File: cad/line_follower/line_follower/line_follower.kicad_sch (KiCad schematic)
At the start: 15 parts

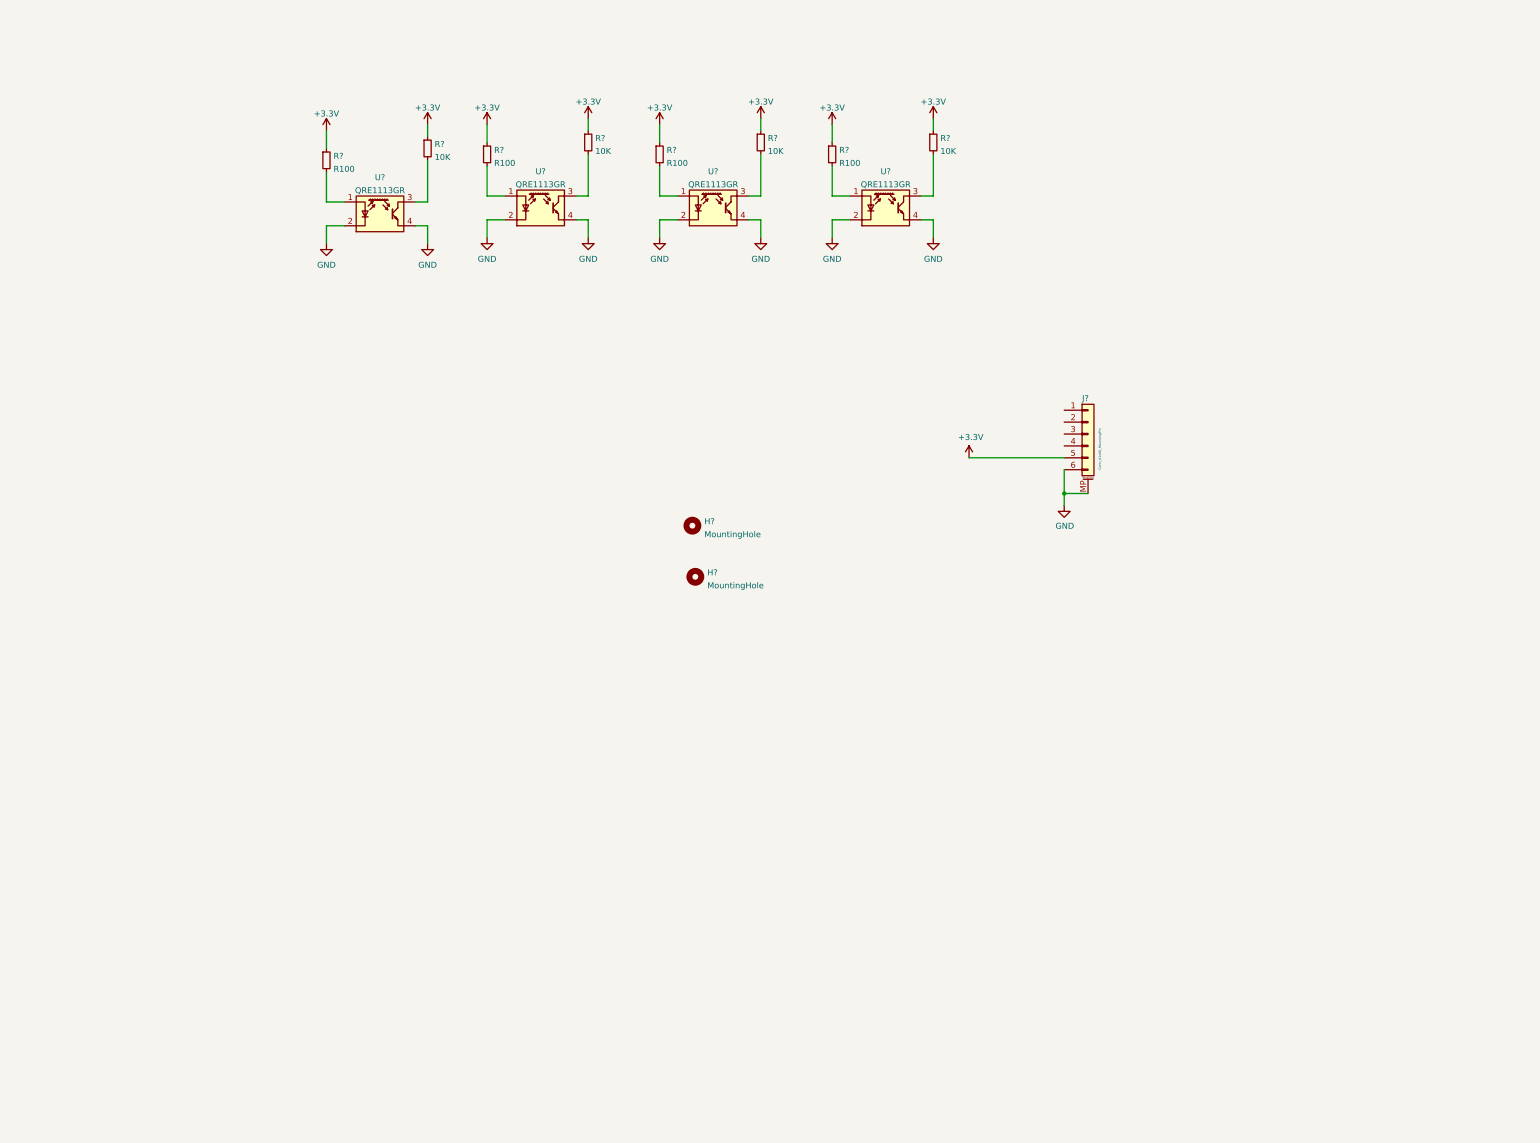
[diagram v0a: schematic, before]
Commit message: Andrew wants what!?!?! 5 more boards???
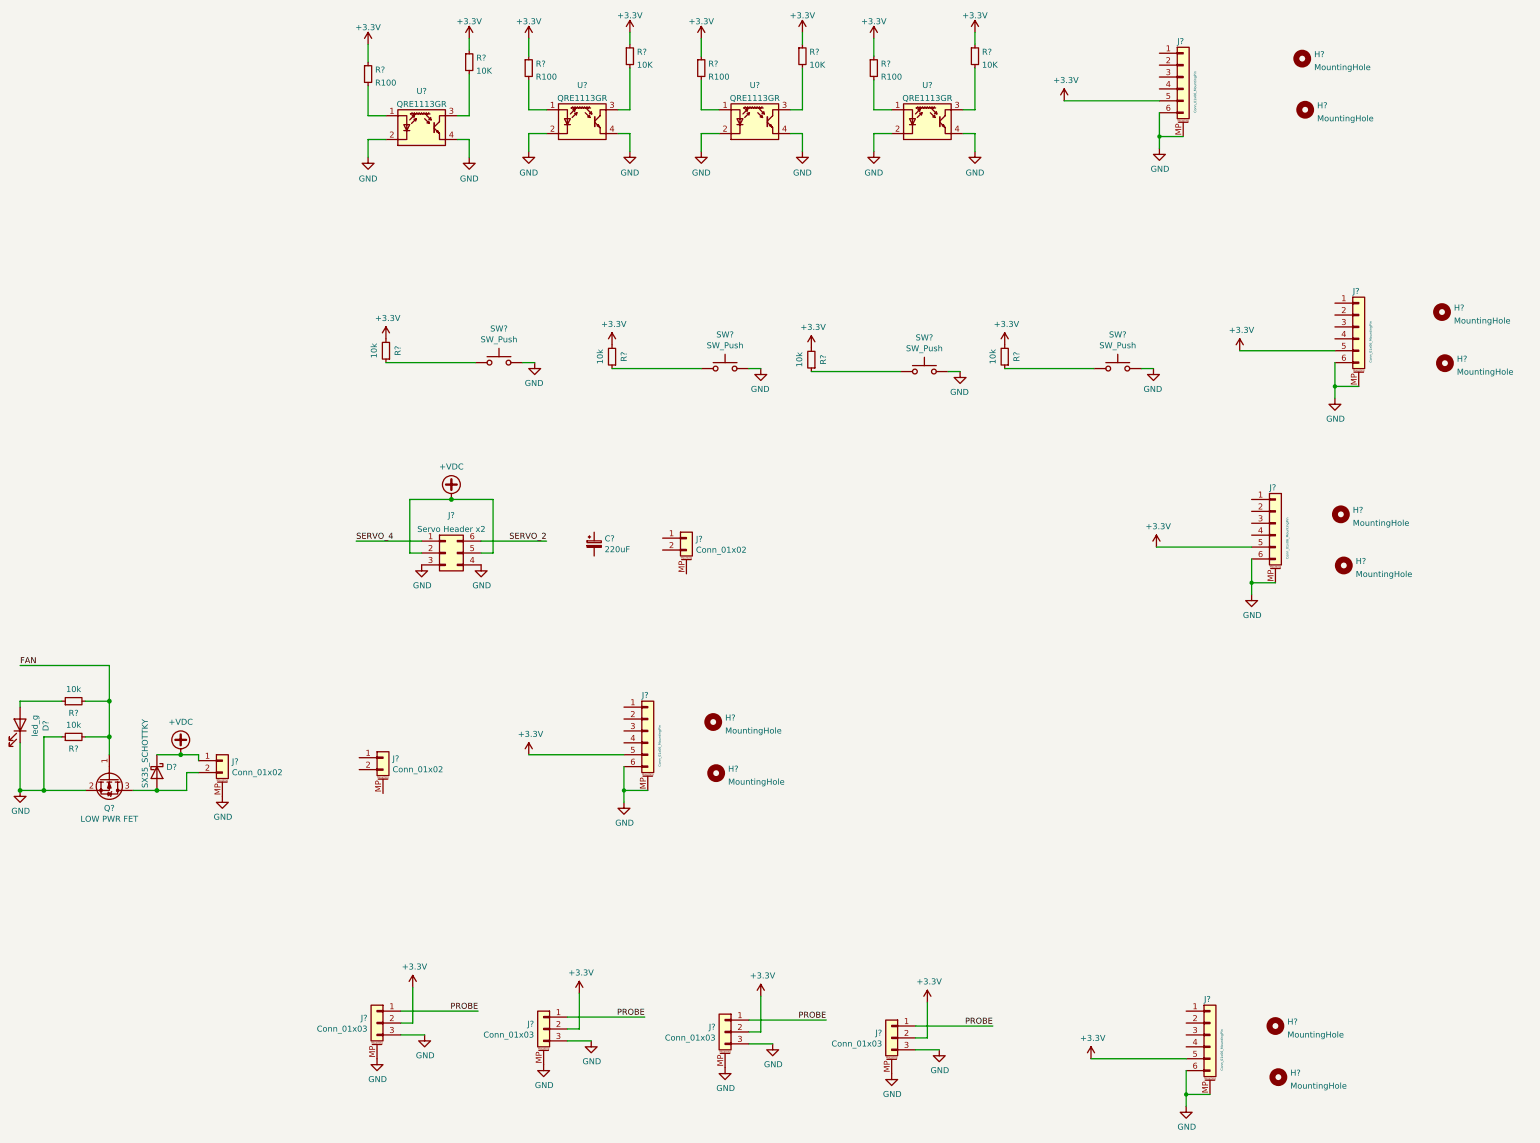
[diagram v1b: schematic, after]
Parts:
- added C?: 220uF, Capacitor_SMD:CP_Elec_10x12.5, symbol Device:CP_Small
- added D?: led_g, LED_SMD:LED_0603_1608Metric, symbol Device:LED
- added D?: SX35_SCHOTTKY, Diode_SMD:D_SMA, symbol Device:D_Schottky
- added H? (x8): MountingHole, MountingHole:MountingHole_3.2mm_M3_ISO14580, symbol Mechanical:MountingHole
- added J? (x4): Conn_01x03, Connector_JST:JST_PH_B3B-PH-SM4-TB_1x03-1MP_P2.00mm_Vertical, symbol Connector_Generic_MountingPin:Conn_01x03_MountingPin
- added J?: Servo Header x2, Evezor_extras:PinHeader_2x03_P2.54mm_Vertical_SMD, symbol Connector_Generic:Conn_02x03_Counter_Clockwise
- added J? (x4): Conn_01x06_MountingPin, Connector_FFC-FPC:TE_84952-6_1x06-1MP_P1.0mm_Horizontal, symbol Connector_Generic_MountingPin:Conn_01x06_MountingPin
- added J? (x3): Conn_01x02, Evezor_extras:CONN_JST_XH_2_VERTICAL, symbol Connector_Generic_MountingPin:Conn_01x02_MountingPin
- added Q?: LOW PWR FET, Package_TO_SOT_SMD:SOT-23, symbol Device:Q_NMOS_GSD
- added R? (x6): 10k, Resistor_SMD:R_0603_1608Metric, symbol Device:R_Small
- added SW? (x4): SW_Push, EvezorLIB:SWITCH_2x3_SMD_TACTILE_GREEN, symbol Switch:SW_Push
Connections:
- net +3V3: now also J?.2 (Pin_2), J?.2 (Pin_2), J?.2 (Pin_2), J?.2 (Pin_2), J?.5 (Pin_5), J?.5 (Pin_5), J?.5 (Pin_5), J?.5 (Pin_5), R?.2, R?.2, R?.2, R?.2
- net GND: now also D?.1 (K), J?.3 (Pin_3), J?.3 (Pin_3), J?.3 (Pin_3), J?.3 (Pin_3), J?.3 (Pin_3), J?.4 (Pin_4), J?.6 (Pin_6), J?.6 (Pin_6), J?.6 (Pin_6), J?.6 (Pin_6), J?.MP (MountPin), J?.MP (MountPin), J?.MP (MountPin), J?.MP (MountPin), J?.MP (MountPin), J?.MP (MountPin), J?.MP (MountPin), J?.MP (MountPin), J?.MP (MountPin), Q?.2 (S), R?.1, SW?.2, SW?.2, SW?.2, SW?.2
- new net: R?.1, SW?.1 (x4)
- new net: D?.2 (A), R?.1
- new net: D?.2 (A), J?.2 (Pin_2), Q?.3 (D)
- new net +VDC: D?.1 (K), J?.1 (Pin_1), J?.2 (Pin_2), J?.5 (Pin_5)
- new net FAN: Q?.1 (G), R?.2, R?.2
- new net PROBE: J?.1 (Pin_1), J?.1 (Pin_1), J?.1 (Pin_1), J?.1 (Pin_1)
- new net SERVO_2: J?.6 (Pin_6)
- new net SERVO_4: J?.1 (Pin_1)
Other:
- moved on the sheet: H?, J?, R?, U?

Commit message: Half of the 2nd floor built, remodeling in progress
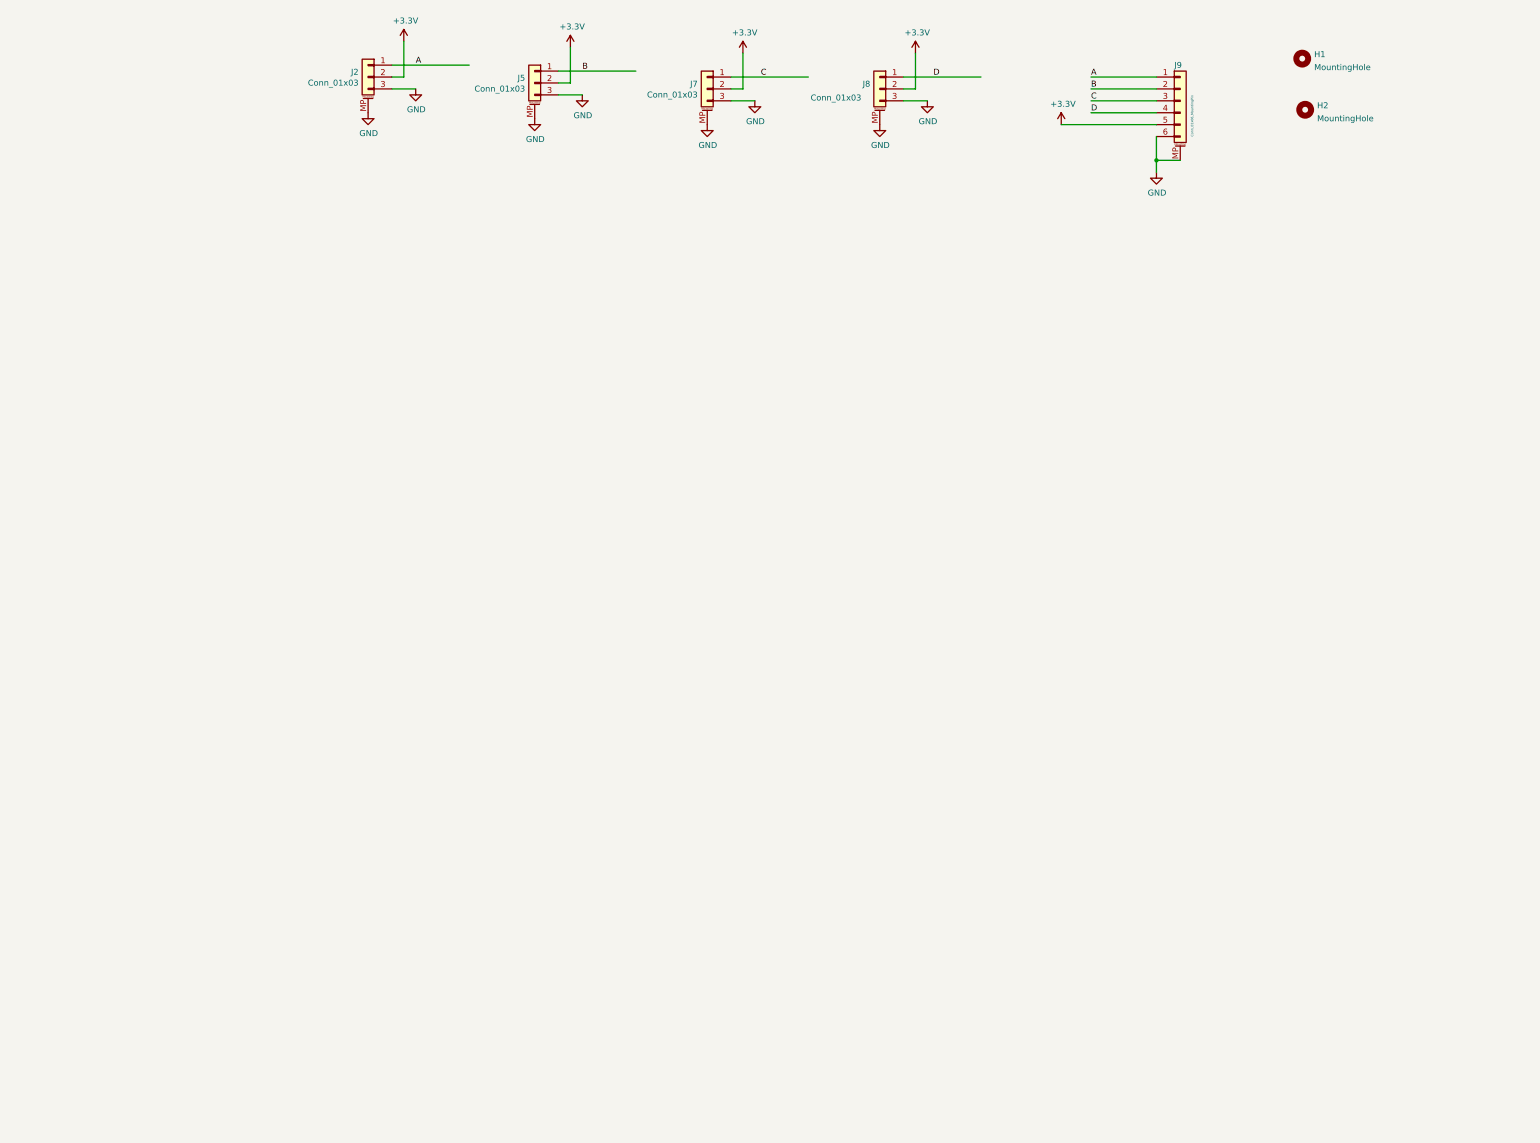
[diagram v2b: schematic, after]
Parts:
- removed C?: 220uF, Capacitor_SMD:CP_Elec_10x12.5, symbol Device:CP_Small
- removed D?: led_g, LED_SMD:LED_0603_1608Metric, symbol Device:LED
- removed D?: SX35_SCHOTTKY, Diode_SMD:D_SMA, symbol Device:D_Schottky
- removed H? (x8): MountingHole, MountingHole:MountingHole_3.2mm_M3_ISO14580, symbol Mechanical:MountingHole
- removed J?: Servo Header x2, Evezor_extras:PinHeader_2x03_P2.54mm_Vertical_SMD, symbol Connector_Generic:Conn_02x03_Counter_Clockwise
- removed J? (x4): Conn_01x06_MountingPin, Connector_FFC-FPC:TE_84952-6_1x06-1MP_P1.0mm_Horizontal, symbol Connector_Generic_MountingPin:Conn_01x06_MountingPin
- removed J? (x3): Conn_01x02, Evezor_extras:CONN_JST_XH_2_VERTICAL, symbol Connector_Generic_MountingPin:Conn_01x02_MountingPin
- removed Q?: LOW PWR FET, Package_TO_SOT_SMD:SOT-23, symbol Device:Q_NMOS_GSD
- removed R? (x6): 10k, Resistor_SMD:R_0603_1608Metric, symbol Device:R_Small
- removed R? (x4): 10K, Resistor_SMD:R_0603_1608Metric, symbol Device:R_Small
- removed R? (x4): R100, Resistor_SMD:R_0603_1608Metric, symbol Device:R_Small
- removed SW? (x4): SW_Push, EvezorLIB:SWITCH_2x3_SMD_TACTILE_GREEN, symbol Switch:SW_Push
- removed U? (x4): QRE1113GR, OptoDevice:OnSemi_CASE100CY, symbol Sensor_Proximity:QRE1113
- gave numbers to parts that had none: 7
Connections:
- net A: now reaches J9.1 (Pin_1)
- net A: now also J2.1 (Pin_1)
- net B: now reaches J9.2 (Pin_2)
- net B: now also J5.1 (Pin_1)
- net C: now reaches J9.3 (Pin_3)
- net C: now also J7.1 (Pin_1)
- net D: now reaches J9.4 (Pin_4)
- net D: now also J8.1 (Pin_1)
- removed net PROBE: J2.1 (Pin_1), J5.1 (Pin_1), J7.1 (Pin_1), J8.1 (Pin_1)
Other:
- moved on the sheet: J2, J5, J7, J8, J9

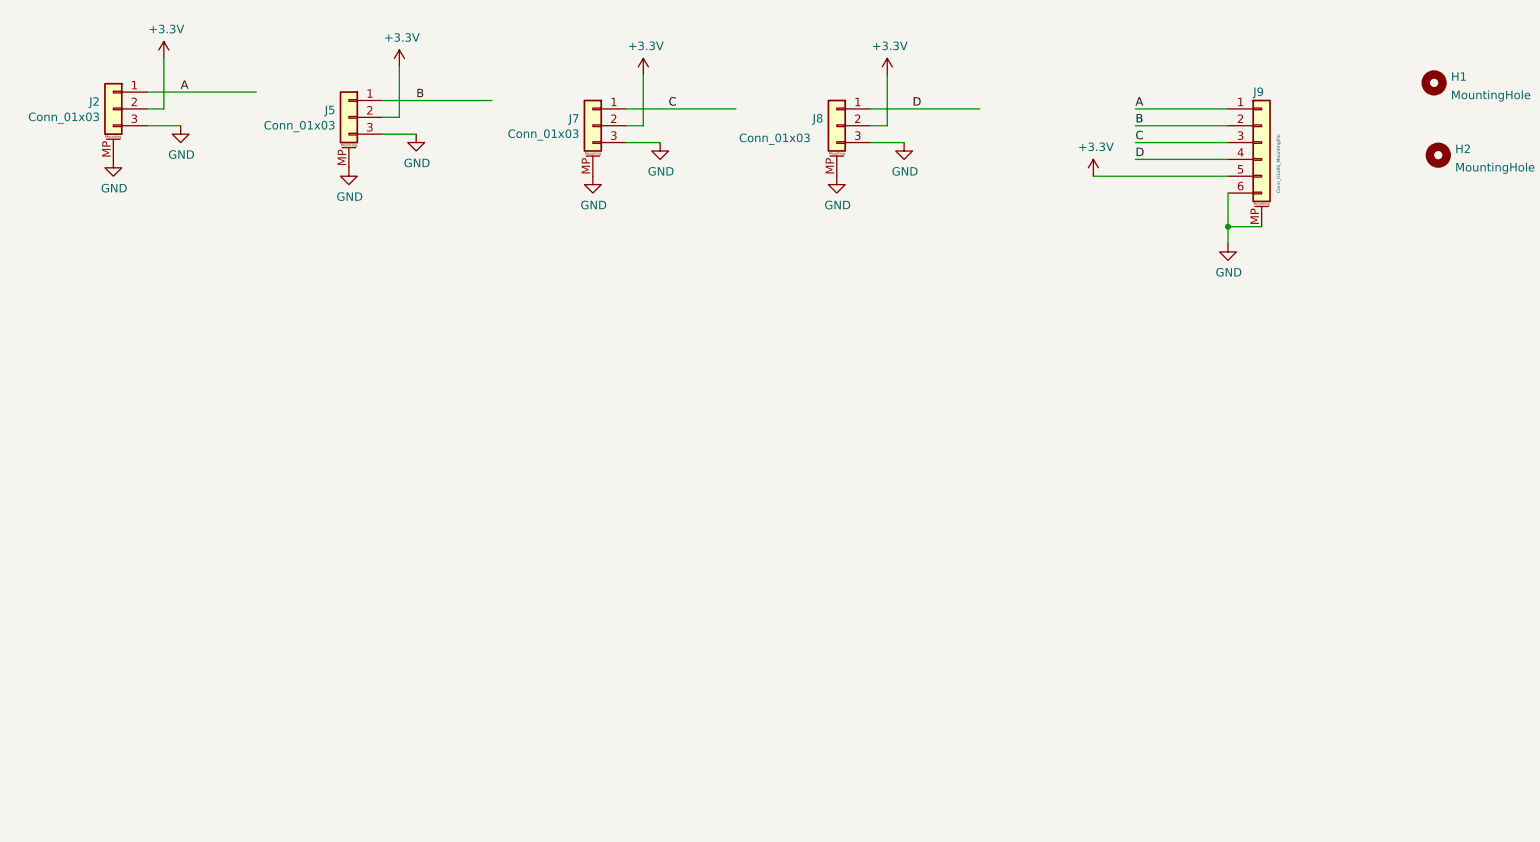
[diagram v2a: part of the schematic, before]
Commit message: Mega monster huge scary big board 4.0 big scary there's like 4 pieces but its actually not that scary huge hugh mungus big board also mousey bites
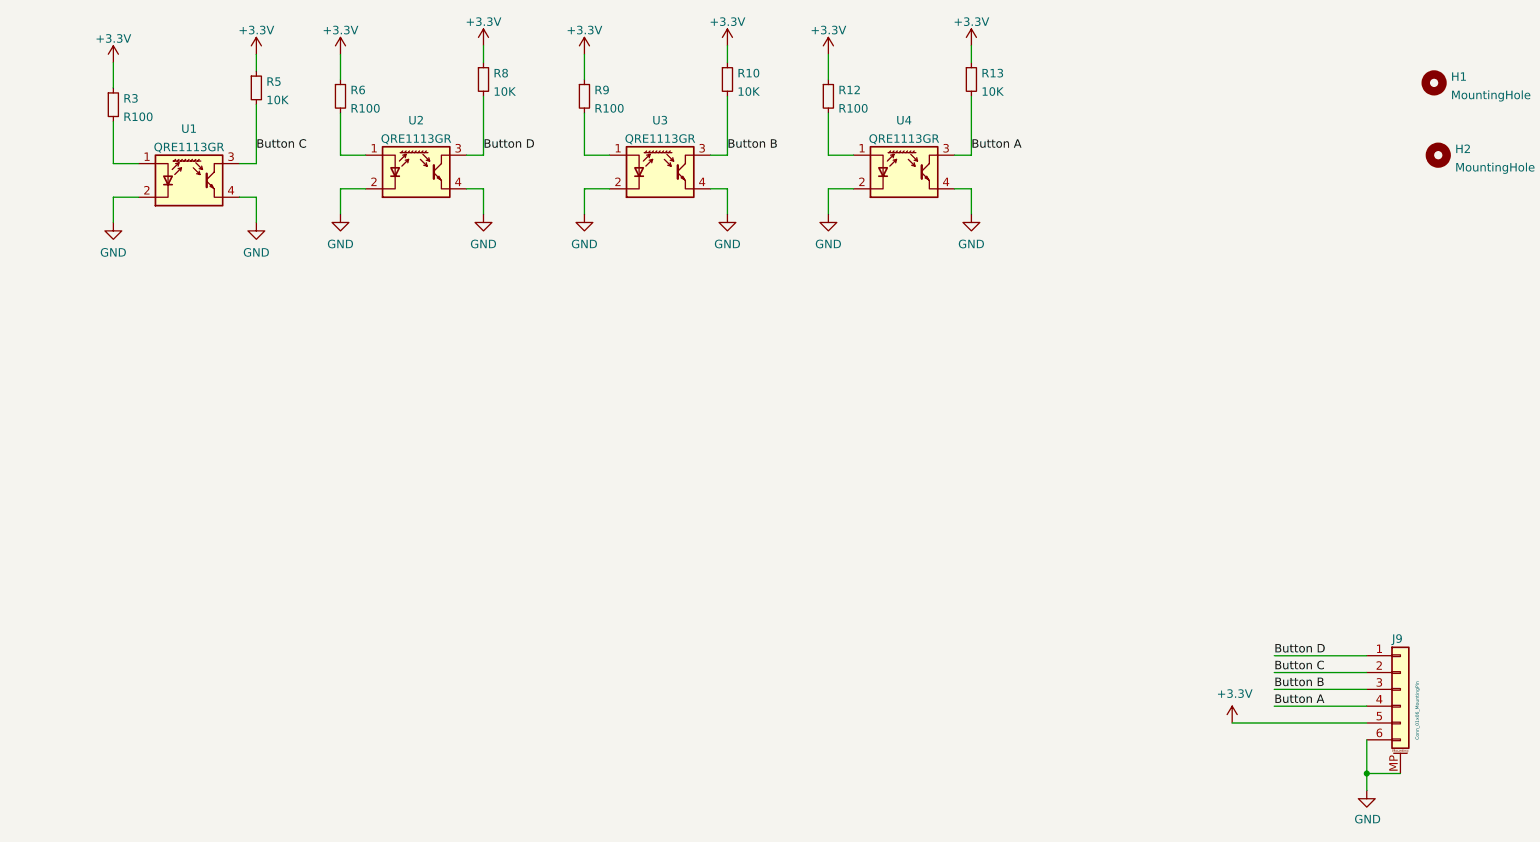
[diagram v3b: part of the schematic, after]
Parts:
- removed J2, J5, J7, J8: Conn_01x03, Connector_JST:JST_PH_B3B-PH-SM4-TB_1x03-1MP_P2.00mm_Vertical, symbol Connector_Generic_MountingPin:Conn_01x03_MountingPin
- added R10, R13, R5, R8: 10K, Resistor_SMD:R_0603_1608Metric, symbol Device:R_Small
- added R12, R3, R6, R9: R100, Resistor_SMD:R_0603_1608Metric, symbol Device:R_Small
- added U1, U2, U3, U4: QRE1113GR, OptoDevice:OnSemi_CASE100CY, symbol Sensor_Proximity:QRE1113
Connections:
- net +3V3: now also R10.1, R12.1, R13.1, R3.1, R5.1, R6.1, R8.1, R9.1
- net GND: now also U1.2 (K), U1.4, U2.2 (K), U2.4, U3.2 (K), U3.4, U4.2 (K), U4.4
- net A renamed Button D
- net Button D: now also R8.2, U2.3
- net B renamed Button C
- net Button C: now also R5.2, U1.3
- net C renamed Button B
- net Button B: now also R10.2, U3.3
- net D renamed Button A
- net Button A: now also R13.2, U4.3
- new net: R9.2, U3.1 (A)
- new net: R6.2, U2.1 (A)
- new net: R12.2, U4.1 (A)
- new net: R3.2, U1.1 (A)
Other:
- moved on the sheet: J9
